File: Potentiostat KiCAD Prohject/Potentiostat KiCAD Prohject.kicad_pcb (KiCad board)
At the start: 2 copper layers, 46 parts, among them J2 USB_C_Receptacle_USB2.0, K1 DIPxx-1Axx-12xD, SW1 Reset, SW2 Boot, U1 OPA2277, U10 ADS1115IDGS, U11 MCP4725xxx-xCH, U13 LD1117S33TR_SOT223, U14 ESP32-S2-SOLO, U2 TL074, U4 OPA2277, U5 INA128, U6 MCP4725xxx-xCH, U7 INA128, U8 REF3033, U9 INA128

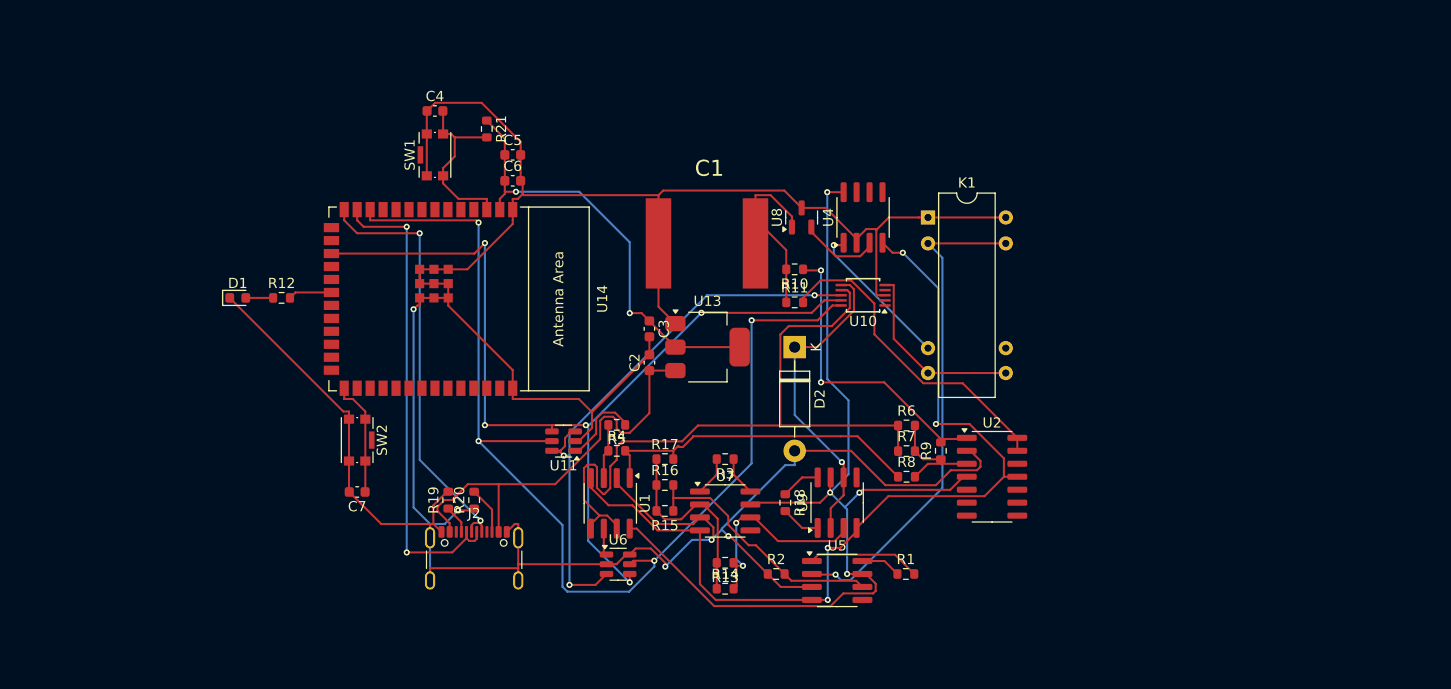
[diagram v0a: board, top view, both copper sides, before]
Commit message: we're so back
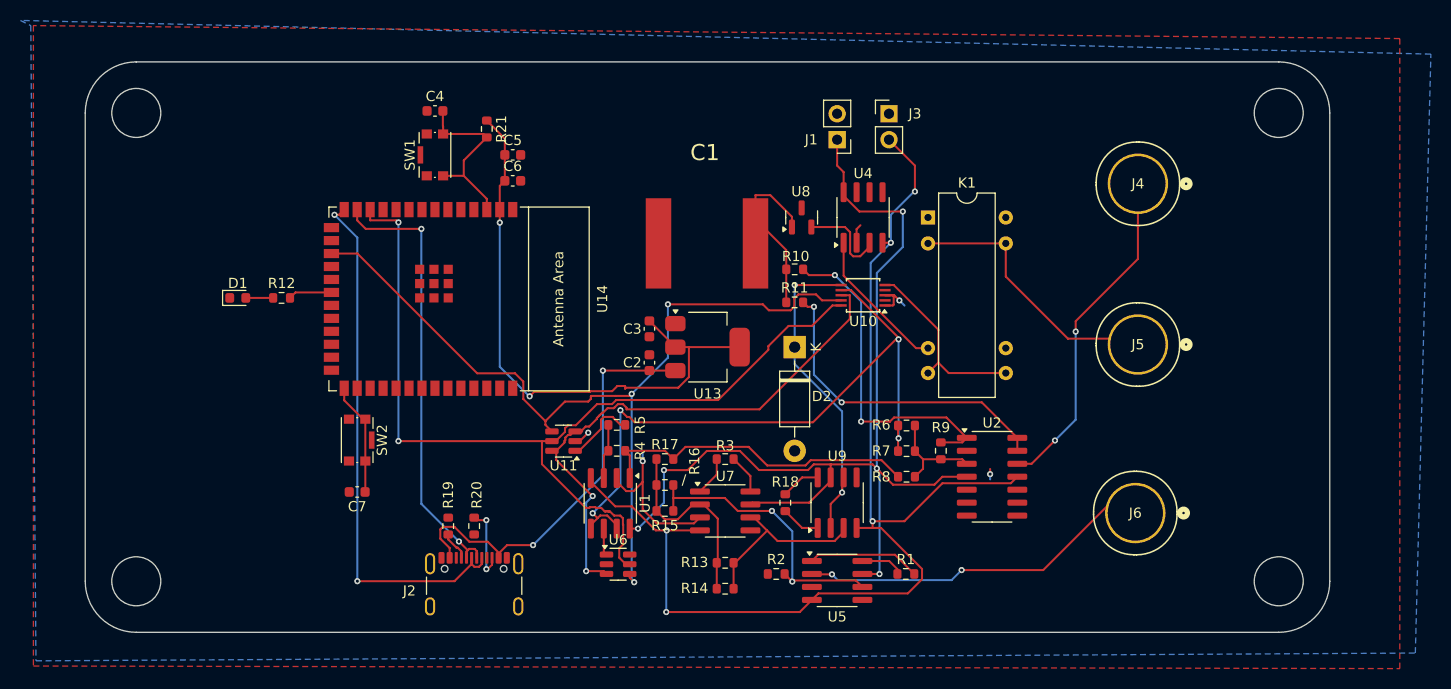
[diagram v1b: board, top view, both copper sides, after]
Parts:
- added J1: Conn_01x02_Pin, Connector_PinHeader_2.54mm:PinHeader_1x02_P2.54mm_Vertical, F.Cu at (190.5, 61.0)
- added J3: Conn_01x02_Pin, Connector_PinHeader_2.54mm:PinHeader_1x02_P2.54mm_Vertical, F.Cu at (195.6, 58.4)
- added J4: Reference, i made this:CONN_575-8_KEY, F.Cu at (220.0, 65.3)
- added J5: Working, i made this:CONN_575-8_KEY, F.Cu at (220.0, 81.0)
- added J6: Working, i made this:CONN_575-8_KEY, F.Cu at (219.7, 97.5)
- U10: value ADS1115IDGS -> ADS1115
- U11: value MCP4725xxx-xCH -> MCP4725
- moved J2 2.54 mm to (154.9, 105.6)
- moved R19 2.54 mm to (152.4, 98.8)
- moved R20 2.54 mm to (154.9, 98.8)
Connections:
- K1 pad 13: /Working Electrode -> Net-(J5-Pin_1)
- K1 pad 2: /Working Electrode -> Net-(J5-Pin_1)
- U10 pad 1: unconnected-(U10-ADDR-Pad1) -> GND
- U2 pad 12: /Reference Electrode -> Net-(J4-Pin_1)
- U5 pad 2: /Working Electrode -> Net-(J6-Pin_1)
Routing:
- net GND: track 323.6 -> 25.0 mm, vias 5 -> 4
- net /Working Electrode: track 48.9 -> 0.00 mm, vias 1 -> 0
- net Net-(J6-Pin_1): track 0.00 -> 35.9 mm, vias 0 -> 2
- net Net-(J4-Pin_1): track 0.00 -> 33.1 mm, vias 0 -> 2
- net Net-(J5-Pin_1): track 0.00 -> 26.9 mm
- net -9V: track 89.1 -> 114.3 mm, vias 4 -> 5
- net /I2C_SCL: track 108.2 -> 92.4 mm, vias 4 -> 2
- net +3.3V: track 43.0 -> 58.8 mm
- net /D+: track 42.4 -> 52.3 mm
- net +9V: track 96.0 -> 101.2 mm, vias 4 -> 5
- net /I2C_SDA: track 91.8 -> 88.1 mm, vias 5 -> 3
- net Net-(R15-Pad1): track 25.2 -> 28.7 mm, vias 0 -> 2
- net /D-: track 47.0 -> 43.5 mm
- net Net-(R10-Pad1): track 29.7 -> 32.8 mm
- net Net-(J2-CC2): track 4.66 -> 7.51 mm, vias 0 -> 2
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- added copper zone on B.Cu, net GND
- added copper zone on F.Cu, net GND
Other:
- board outline added: 121.9 x 55.9 mm
- board text added: "/"
